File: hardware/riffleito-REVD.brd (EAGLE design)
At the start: 74.6 x 18 mm, 31 parts, among them IC1 ATMEGA328P, IC2 24AA128SN, IC4 MCP1700-33, X1 16 MHz

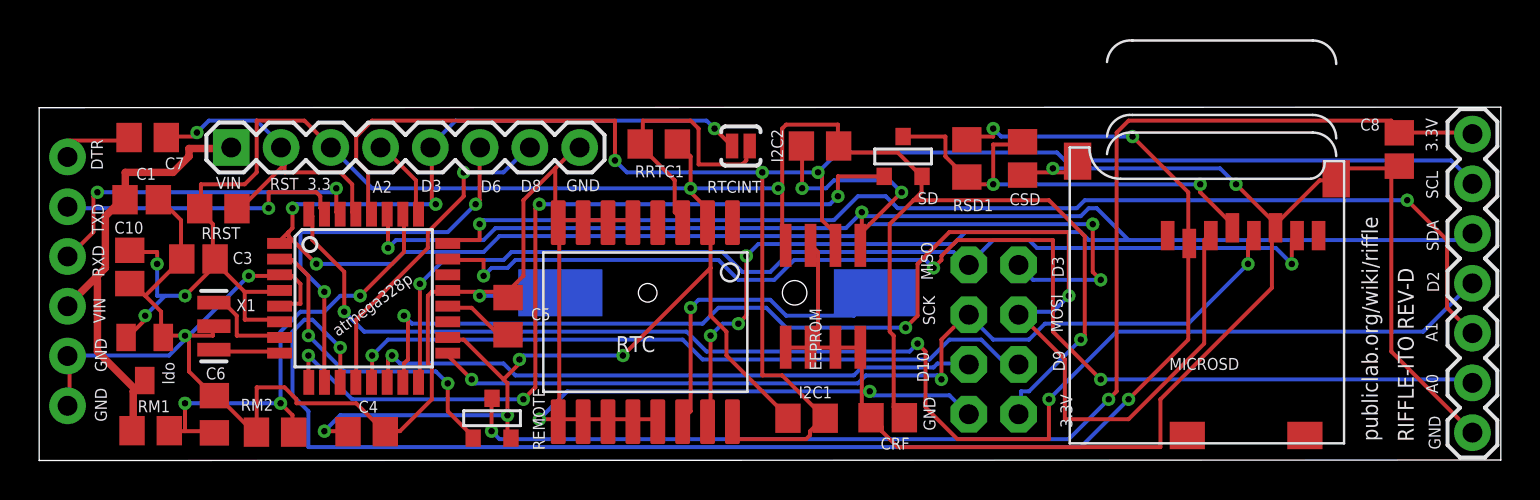
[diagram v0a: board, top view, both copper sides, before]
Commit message: update
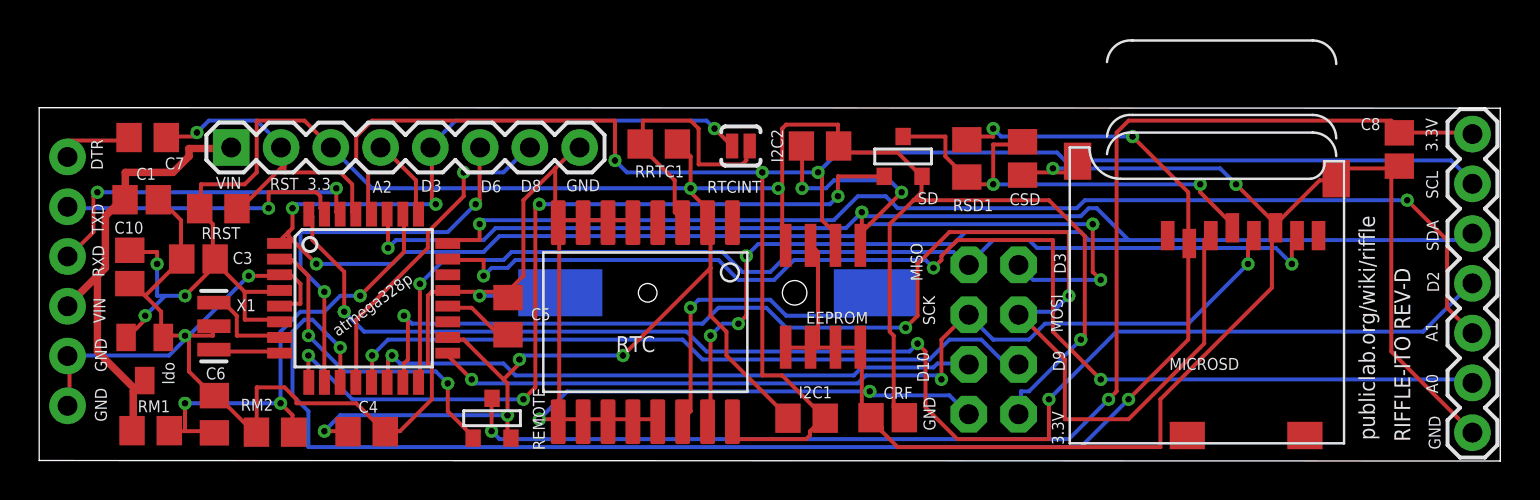
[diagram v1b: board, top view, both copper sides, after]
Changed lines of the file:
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@@
 <plain>
 <wire x1="0.0762" y1="-0.0762" x2="0.0762" y2="17.9324" width="0" layer="20"/>
-<wire x1="0.0762" y1="17.9324" x2="74.676" y2="17.9578" width="0" layer="20"/>
-<wire x1="74.676" y1="17.9578" x2="74.676" y2="-0.0508" width="0" layer="20"/>
-<wire x1="74.676" y1="-0.0508" x2="0.0762" y2="-0.0762" width="0" layer="20"/>
+<wire x1="0.0762" y1="17.9324" x2="74.6506" y2="17.907" width="0" layer="20"/>
+<wire x1="74.6506" y1="17.907" x2="74.6506" y2="-0.1016" width="0" layer="20"/>
+<wire x1="74.6506" y1="-0.1016" x2="0.0762" y2="-0.0762" width="0" layer="20"/>
 <text x="6.3754" y="4.953" size="0.6096" layer="21" rot="R270">ldo</text>
-<text x="39.3954" y="7.6962" size="0.6096" layer="21" rot="R270">EEPROM</text>
+<text x="39.2176" y="6.9088" size="0.6096" layer="21">EEPROM</text>
 <text x="22.606" y="13.6144" size="0.6096" layer="21">D6</text>
 <text x="28.702" y="14.2748" size="0.6096" layer="21" rot="R180">GND</text>
@@
 <text x="44.8818" y="5.461" size="0.6096" layer="21" rot="R270">D10</text>
 <text x="45.1866" y="8.3312" size="0.6096" layer="21" rot="R270">SCK</text>
-<text x="45.085" y="11.0744" size="0.6096" layer="21" rot="R270">MISO</text>
-<text x="51.7652" y="10.3378" size="0.6096" layer="21" rot="R270">D3</text>
+<text x="44.5516" y="11.0236" size="0.6096" layer="21" rot="R270">MISO</text>
+<text x="51.8668" y="10.5156" size="0.6096" layer="21" rot="R270">D3</text>
 <text x="51.7144" y="8.4074" size="0.6096" layer="21" rot="R270">MOSI</text>
 <text x="51.816" y="5.5372" size="0.6096" layer="21" rot="R270">D9</text>
-<text x="52.197" y="3.302" size="0.6096" layer="21" rot="R270">3.3V</text>
+<text x="51.7652" y="2.4384" size="0.6096" layer="21" rot="R270">3.3V</text>
 <text x="70.8406" y="17.399" size="0.6096" layer="21" rot="R270">3.3V</text>
 <text x="70.9168" y="9.5758" size="0.6096" layer="21" rot="R270">D2</text>
@@
 <text x="18.8468" y="9.5504" size="0.6096" layer="21" rot="R216">atmega328p</text>
 <text x="69.469" y="5.207" size="0.8128" layer="22" rot="MR0">publicab.org/wiki/riffle</text>
-<text x="70.231" y="0.889" size="0.8128" layer="21" rot="R90">RIFFLE-ITO REV-D</text>
+<text x="70.0532" y="0.889" size="0.8128" layer="21" rot="R90">RIFFLE-ITO REV-D</text>
 <text x="69.4182" y="6.1468" size="0.8128" layer="22" rot="MR0">RIFFLE-IT REV-D</text>
 <text x="69.4436" y="3.9624" size="0.8128" layer="22" rot="MR0">CERN OHL v1.2</text>
@@
 <wire x1="71.7296" y1="0.6858" x2="44.7294" y2="0.6604" width="0.4064" layer="22"/>
 <wire x1="44.7294" y1="0.6604" x2="44.7294" y2="15.24" width="0.4064" layer="22"/>
-<text x="66.548" y="12.7" size="0.8128" layer="22" rot="MR0">&lt;&lt;nordic RF24&gt;&gt;</text>
+<text x="66.3702" y="12.065" size="0.8128" layer="22" rot="MR0">&lt;&lt;nordic RF24&gt;&gt;</text>
 <text x="45.7454" y="3.2004" size="0.6096" layer="22" rot="MR270">GND</text>
 <wire x1="46.1264" y1="0.6604" x2="46.1264" y2="11.176" width="0.4064" layer="22"/>
@@
 <text x="19.558" y="13.6398" size="0.6096" layer="21">D3</text>
 <text x="70.866" y="4.3434" size="0.6096" layer="21" rot="R270">A0</text>
-<text x="68.4022" y="0.9144" size="0.8128" layer="21" rot="R90">publiclab.org/wiki/riffle</text>
+<text x="68.2498" y="0.9652" size="0.8128" layer="21" rot="R90">publiclab.org/wiki/riffle</text>
 <text x="14.9606" y="14.351" size="0.6096" layer="21" rot="R180">3.3</text>
 </plain>
@@
 </element>
 <element name="C8" library="resistor" package="C0805" value=".1u" x="69.4944" y="15.7988" smashed="yes" rot="R90">
-<attribute name="NAME" x="68.5038" y="17.3736" size="0.6096" layer="25" rot="R180"/>
+<attribute name="NAME" x="68.5292" y="17.399" size="0.6096" layer="25" rot="R180"/>
 <attribute name="VALUE" x="71.7804" y="14.9098" size="1.27" layer="27" rot="R90"/>
 </element>
@@
 </element>
 <element name="CRF" library="resistor" package="C0805" value="100u" x="43.3832" y="2.1082" smashed="yes" rot="R180">
-<attribute name="NAME" x="44.5008" y="1.0922" size="0.6096" layer="25" rot="R180"/>
+<attribute name="NAME" x="44.6532" y="3.683" size="0.6096" layer="25" rot="R180"/>
 <attribute name="VALUE" x="44.2722" y="4.3942" size="1.27" layer="27" rot="R180"/>
 </element>
